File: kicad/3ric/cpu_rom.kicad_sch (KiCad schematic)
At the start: 13 parts, among them J1_AND1 74LS08, J3_DEV_DECODE1 74LS154, K1_CPU1 6502-library_65C02S-2, K2_ROM1 SST39SF040

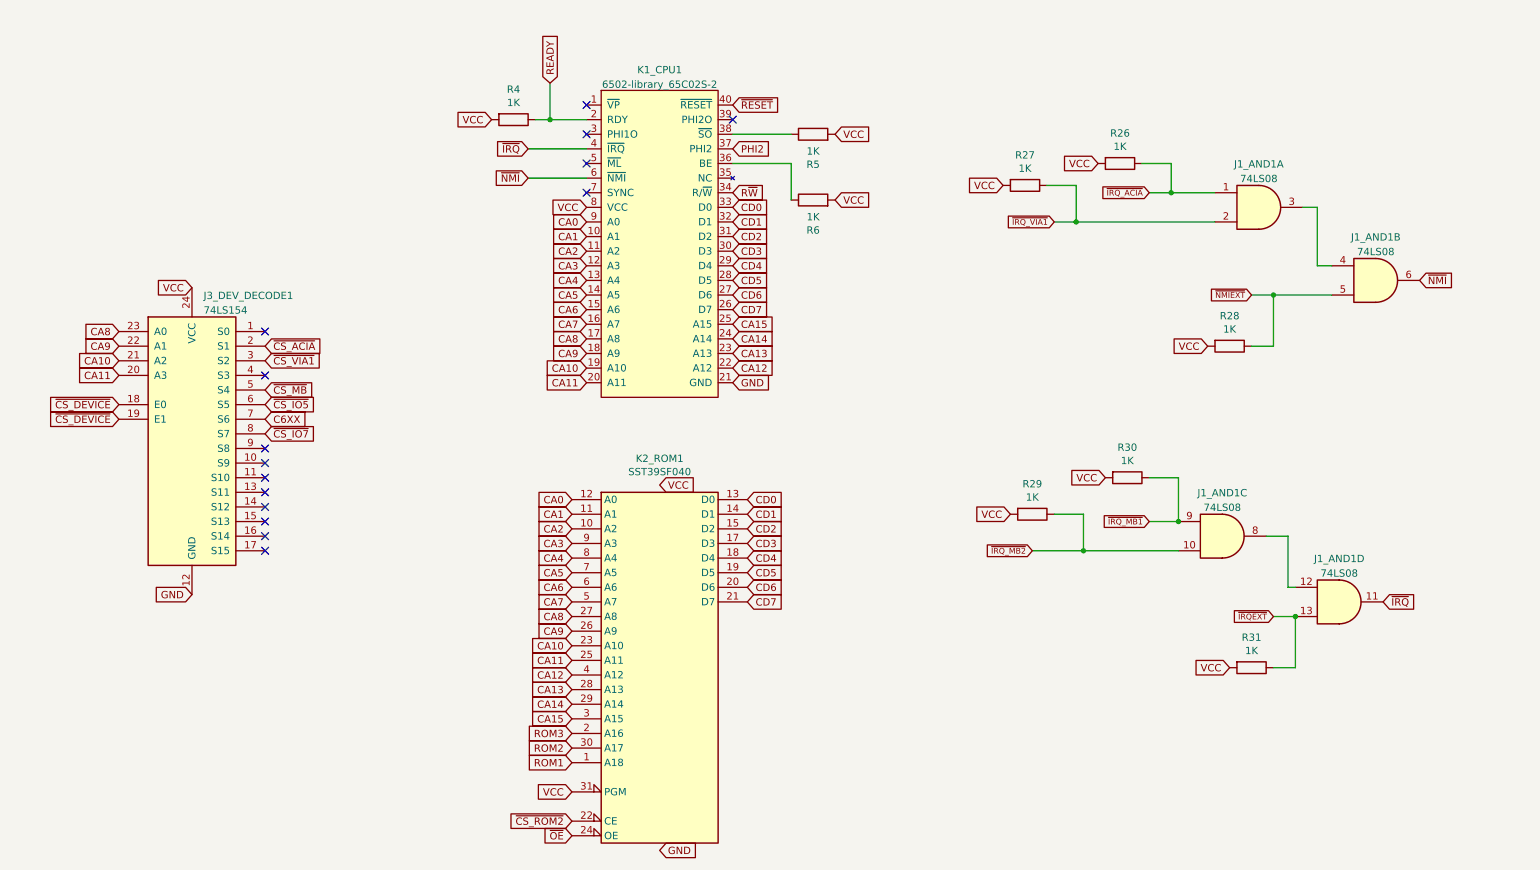
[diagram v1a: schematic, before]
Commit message: v2 pcb
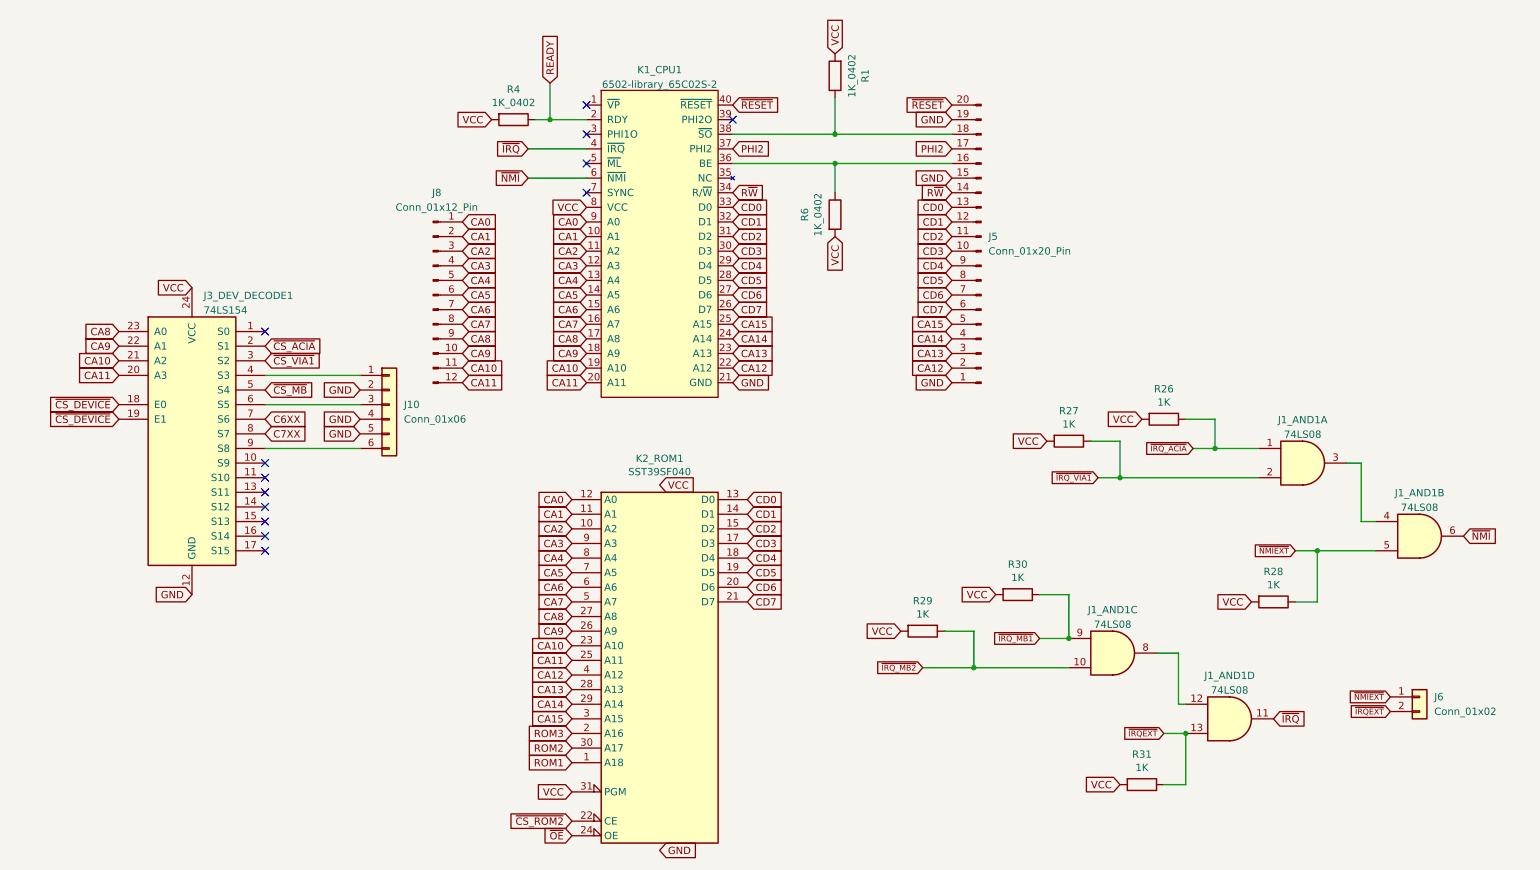
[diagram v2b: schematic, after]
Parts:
- removed R5: 1K, Resistor_SMD:R_0402_1005Metric_Pad0.72x0.64mm_HandSolder, symbol Device:R
- added J10: Conn_01x06, Connector_PinHeader_2.54mm:PinHeader_1x06_P2.54mm_Vertical, symbol Connector_Generic:Conn_01x06
- added J5: Conn_01x20_Pin, Connector_PinHeader_2.54mm:PinHeader_1x20_P2.54mm_Vertical, symbol Connector:Conn_01x20_Pin
- added J6: Conn_01x02, Connector_PinHeader_2.54mm:PinHeader_1x02_P2.54mm_Vertical, symbol Connector_Generic:Conn_01x02
- added J8: Conn_01x12_Pin, Connector_PinHeader_2.54mm:PinHeader_1x12_P2.54mm_Vertical, symbol Connector:Conn_01x12_Pin
- added R1: 1K_0402, Resistor_SMD:R_0402_1005Metric_Pad0.72x0.64mm_HandSolder, symbol Device:R
- R4, R6: value 1K -> 1K_0402
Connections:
- net CA0: now also J8.1 (Pin_1)
- net CA1: now also J8.2 (Pin_2)
- net CA10: now also J8.11 (Pin_11)
- net CA11: now also J8.12 (Pin_12)
- net CA12: now also J5.2 (Pin_2)
- net CA13: now also J5.3 (Pin_3)
- net CA14: now also J5.4 (Pin_4)
- net CA15: now also J5.5 (Pin_5)
- net CA2: now also J8.3 (Pin_3)
- net CA3: now also J8.4 (Pin_4)
- net CA4: now also J8.5 (Pin_5)
- net CA5: now also J8.6 (Pin_6)
- net CA6: now also J8.7 (Pin_7)
- net CA7: now also J8.8 (Pin_8)
- net CA8: now also J8.9 (Pin_9)
- net CA9: now also J8.10 (Pin_10)
- net CD0: now also J5.13 (Pin_13)
- net CD1: now also J5.12 (Pin_12)
- net CD2: now also J5.11 (Pin_11)
- net CD3: now also J5.10 (Pin_10)
- net CD4: now also J5.9 (Pin_9)
- net CD5: now also J5.8 (Pin_8)
- net CD6: now also J5.7 (Pin_7)
- net CD7: now also J5.6 (Pin_6)
- net GND: now also J10.2 (Pin_2), J10.4 (Pin_4), J10.5 (Pin_5), J5.1 (Pin_1), J5.15 (Pin_15), J5.19 (Pin_19)
- net PHI2: now also J5.17 (Pin_17)
- net R~{W}: now also J5.14 (Pin_14)
- net VCC: now also R1.2
- net ~{IRQEXT}: now also J6.2 (Pin_2)
- net ~{NMIEXT}: now also J6.1 (Pin_1)
- net ~{RESET}: now also J5.20 (Pin_20)
- net at K1_CPU1.36 (BE), R6.1: now also J5.16 (Pin_16)
- net at K1_CPU1.38 (~{SO}): now also J5.18 (Pin_18), R1.1
- net at J3_DEV_DECODE1.4 (S3): now also J10.1 (Pin_1)
- net at J3_DEV_DECODE1.9 (S8): now also J10.6 (Pin_6)
- net ~{CS_IO5}: no longer names the net of J3_DEV_DECODE1.6 (S5)
- net ~{CS_IO5}: now also J10.3 (Pin_3)
- net ~{CS_IO7} renamed C7XX
- no-connect marks 15 -> 13
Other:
- moved on the sheet: J1_AND1A, J1_AND1B, J1_AND1C, J1_AND1D, R26, R27, R28, R29, R30, R31, R6
